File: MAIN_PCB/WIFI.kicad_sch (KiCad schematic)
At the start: 25 parts, among them U1 SIT1533AI-H4-DCC-32.768E, U901 MAYA-W166-00B

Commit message: UPDATE
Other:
- company: (none) -> COMPANY_NAME
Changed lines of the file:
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@@
 	(generator "eeschema")
 	(generator_version "9.0")
-	(paper "A4")
+	(paper "A3")
+	(title_block
+		(company "COMPANY_NAME")
+		(comment 1 "Author: Mykola Grodskyi")
+		(comment 2 "Copyright © 2025 Mykola Grodskyi.")
+		(comment 3 "Licensed under CERN-OHL-S v2 (see LICENSE for details)")
+		(comment 4 "PROVIDED \"AS IS\" WITHOUT WARRANTY OF ANY KIND")
+		(comment 5 "Source: github.com/")
+	)
 	(text "Conf settings during boot. internal pull-up exist. \nDon't interfere with it through UART or a pull-down on the input."
 		(exclude_from_sim no)

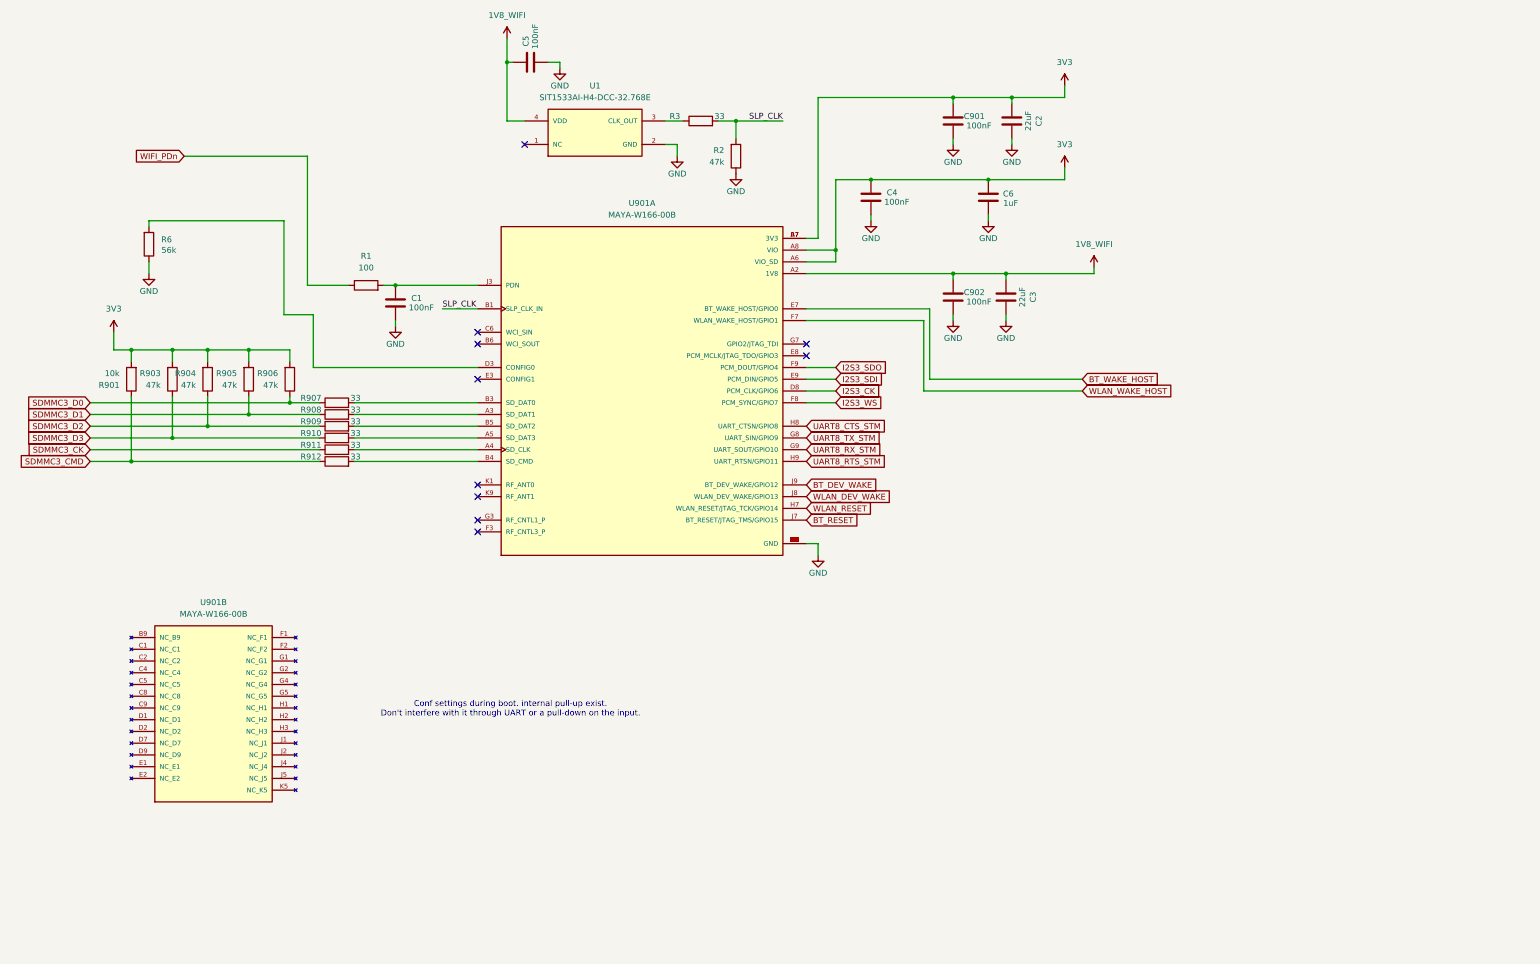
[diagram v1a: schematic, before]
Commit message: UPDATE
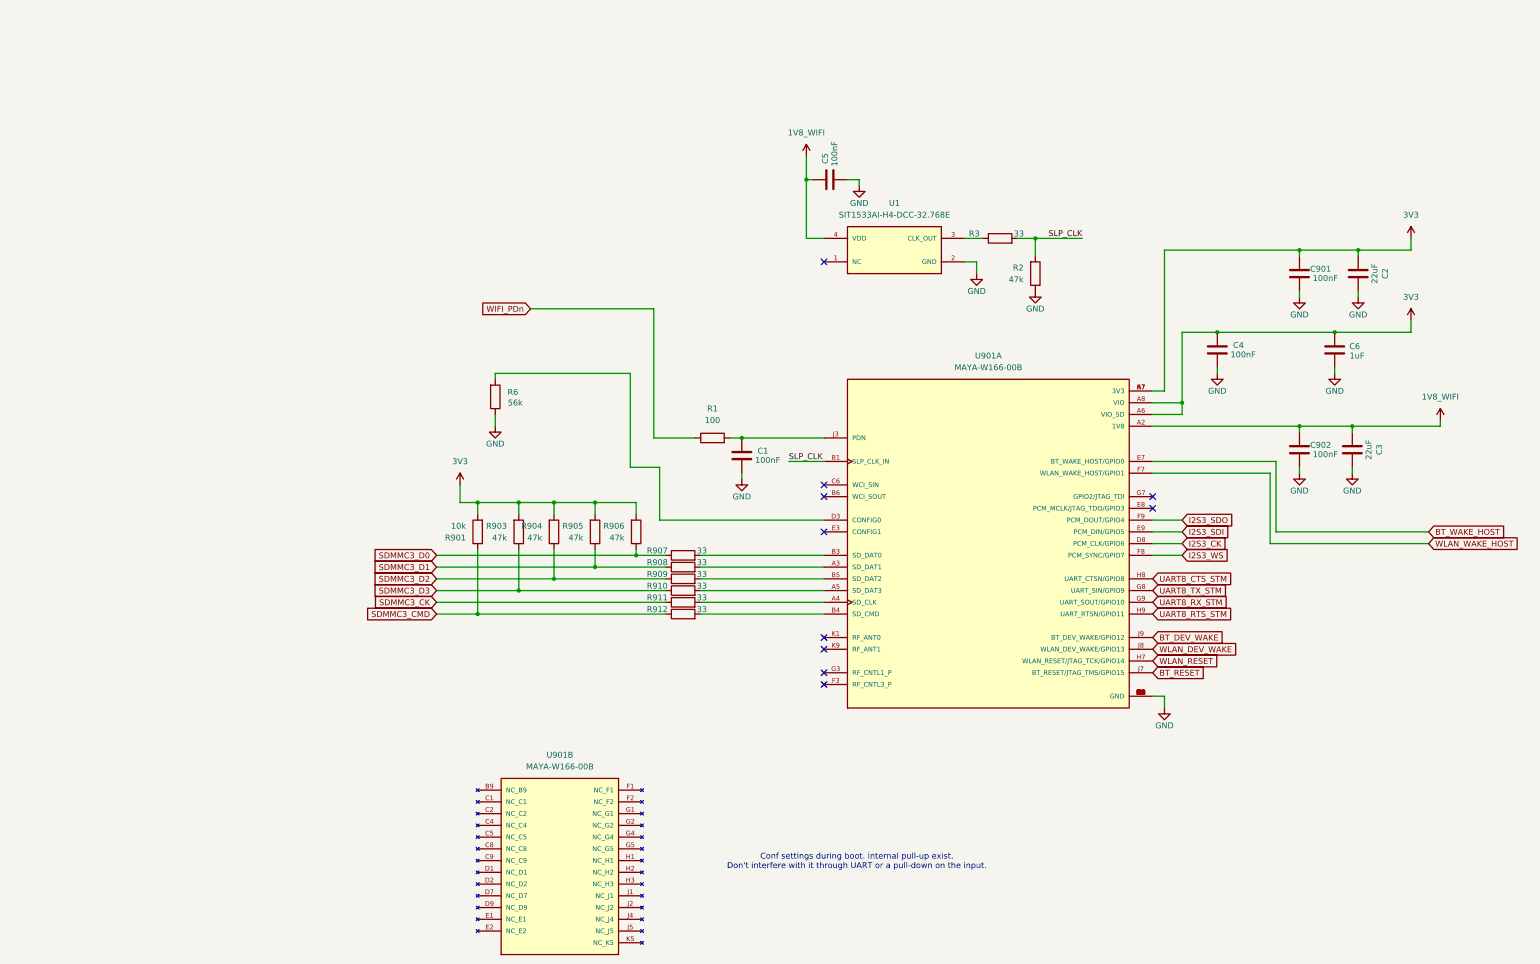
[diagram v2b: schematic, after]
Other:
- moved on the sheet: C1, C2, C3, C4, C5, C6, C901, C902, R1, R2, R3, R6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
